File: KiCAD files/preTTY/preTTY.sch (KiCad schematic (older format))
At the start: 4 parts, among them J1 Power Bus, J2 Signal Buss

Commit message: home
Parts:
- A1: symbol USARTv2-rescue:Arduino_Nano_v3.x-MCU_Module -> preTTY-rescue:Arduino_Nano_v3.x-MCU_Module-USARTv2-rescue
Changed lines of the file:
@@
 EESchema Schematic File Version 4
-LIBS:USARTv2-cache
+LIBS:preTTY-cache
 EELAYER 30 0
 EELAYER END
@@
 Connection ~ 3500 4350
 $Comp
-L USARTv2-rescue:Arduino_Nano_v3.x-MCU_Module A1
+L preTTY-rescue:Arduino_Nano_v3.x-MCU_Module-USARTv2-rescue A1
 U 1 1 60CCDAA2
 P 7250 3700

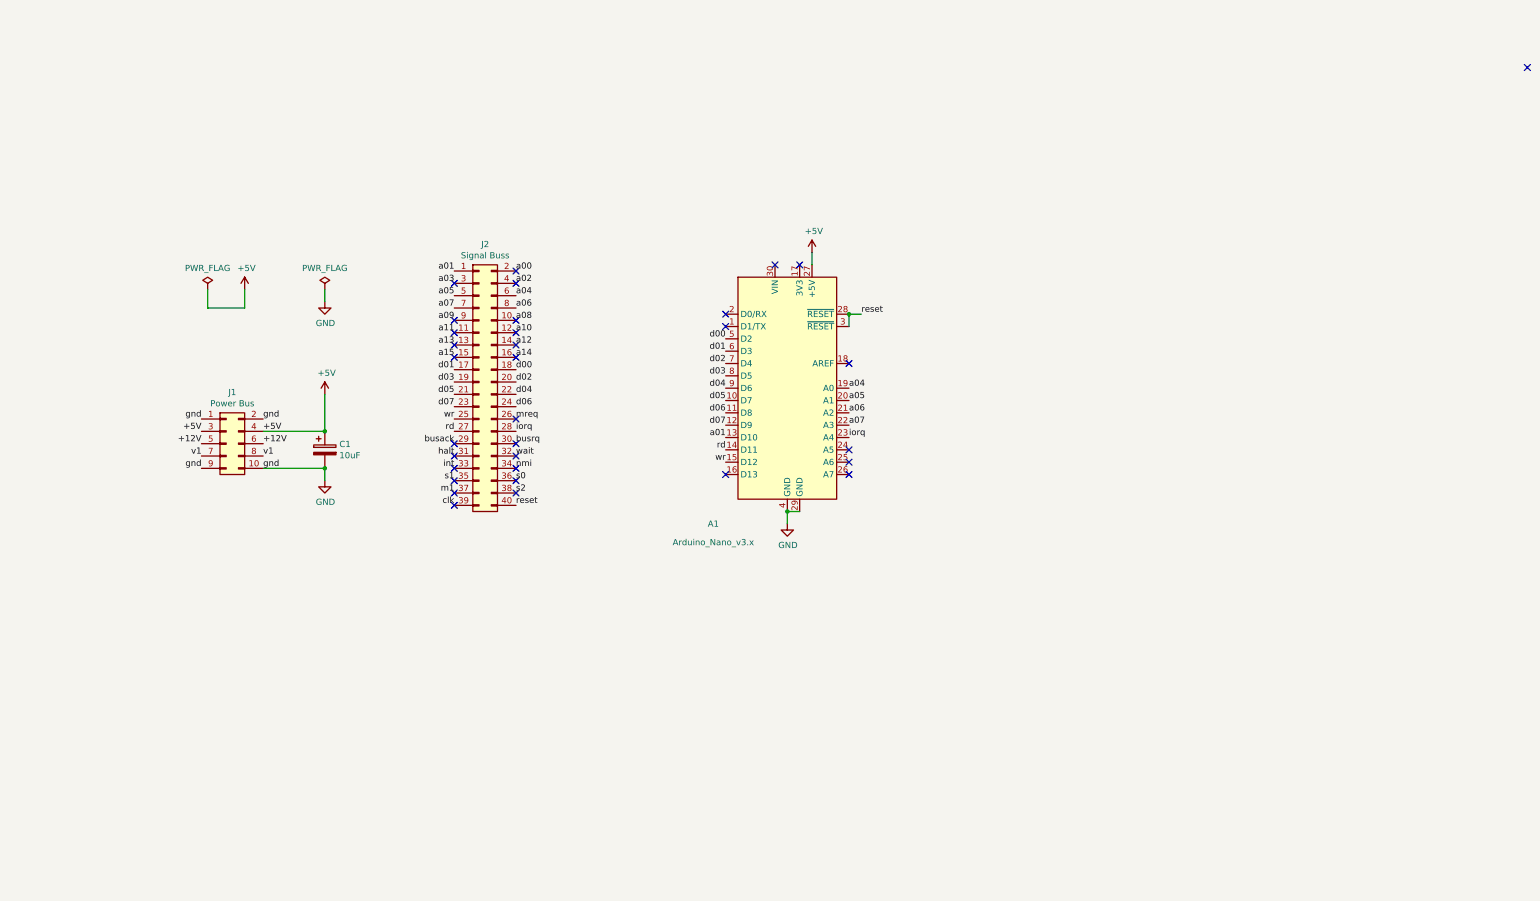
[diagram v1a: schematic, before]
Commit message: office
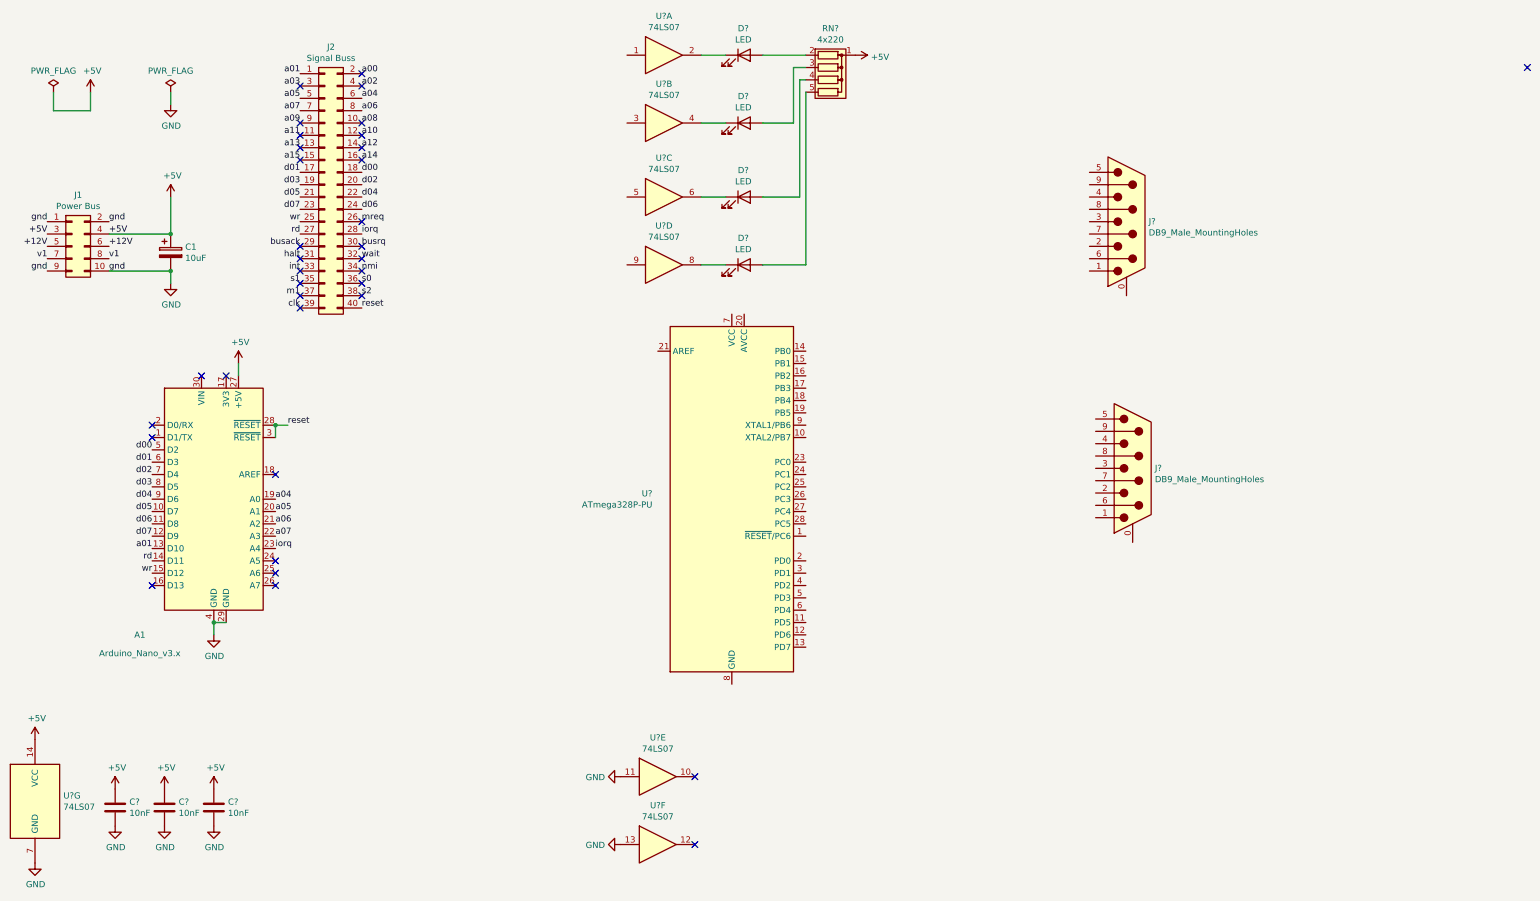
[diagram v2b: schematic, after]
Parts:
- added C? (x3): 10nF, symbol Device:C
- added D? (x4): LED, symbol Device:LED
- added J? (x2): DB9_Male_MountingHoles, symbol Connector:DB9_Male_MountingHoles
- added RN?: 4x220, Resistor_THT:R_Array_SIP5, symbol Device:R_Network04
- added U? (x7): 74LS07, symbol 74xx:74LS07
- added U?: ATmega328P-PU, Package_DIP:DIP-28_W7.62mm, symbol MCU_Microchip_ATmega:ATmega328P-PU
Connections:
- net +5V: now also C?.1, C?.1, C?.1, RN?.1 (common), U?.14 (VCC)
- net GND: now also C?.2, C?.2, C?.2, U?.11, U?.13, U?.7 (GND)
- new net: D?.1 (K), U?.2
- new net: D?.1 (K), U?.4
- new net: D?.1 (K), U?.6
- new net: D?.1 (K), U?.8
- new net: D?.2 (A), RN?.2 (R1)
- new net: D?.2 (A), RN?.3 (R2)
- new net: D?.2 (A), RN?.4 (R3)
- new net: D?.2 (A), RN?.5 (R4)
- new net: U?.22 (GND), U?.8 (GND)
- no-connect marks 33 -> 35
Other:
- moved on the sheet: A1, C1, J1, J2

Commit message: office
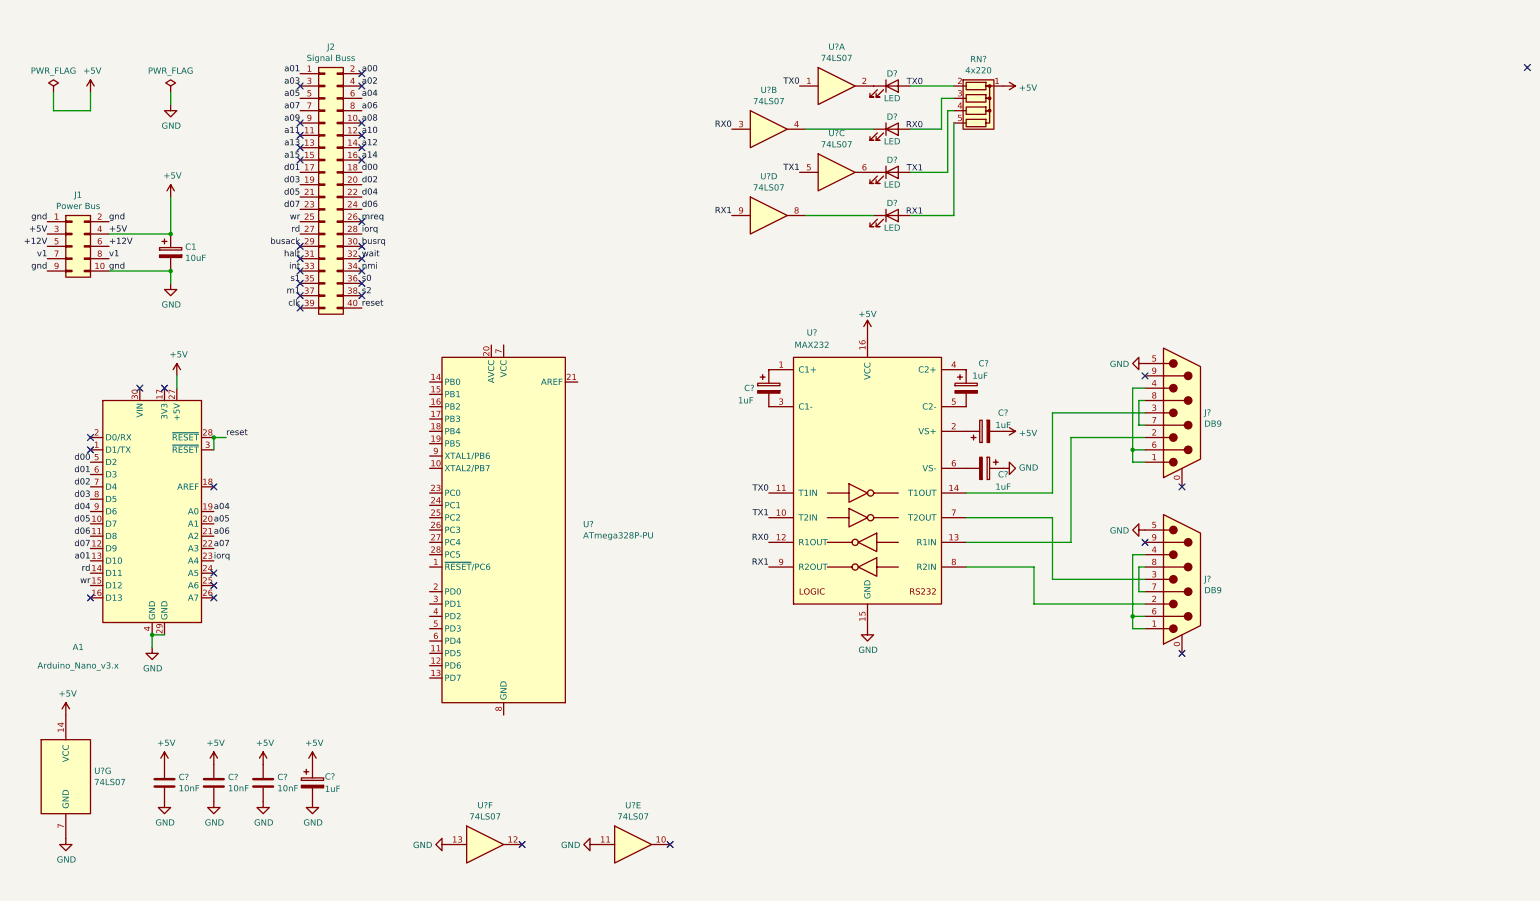
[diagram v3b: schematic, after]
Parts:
- removed J?: DB9_Male_MountingHoles, symbol Connector:DB9_Male_MountingHoles
- added C? (x5): 1uF, symbol Device:CP
- added J?: DB9, symbol Connector:DB9_Male_MountingHoles
- added U?: MAX232, symbol Interface_UART:MAX232
- J?: value DB9_Male_MountingHoles -> DB9
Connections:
- net +5V: now also C?.1, C?.2, U?.16 (VCC)
- net GND: now also J?.5, C?.1, C?.2, J?.5, U?.15 (GND)
- net TX0: now reaches U?.1
- net TX0: now also U?.11 (T1IN)
- net RX0: now reaches U?.3
- net RX0: now also U?.12 (R1OUT)
- net TX1: now reaches U?.5
- net TX1: now also U?.10 (T2IN)
- net RX1: now reaches U?.9
- net RX1: now also U?.9 (R2OUT)
- net at J?.1: now also J?.4, J?.6
- net at J?.2: now also U?.13 (R1IN)
- net at J?.3: now also U?.14 (T1OUT)
- net at J?.7: now also J?.8
- new net: C?.1, U?.1 (C1+)
- new net: C?.1, U?.2 (VS+)
- new net: C?.2, U?.3 (C1-)
- new net: C?.1, U?.4 (C2+)
- new net: C?.2, U?.5 (C2-)
- new net: C?.2, U?.6 (VS-)
- new net: J?.3, U?.7 (T2OUT)
- new net: J?.2, U?.8 (R2IN)
- new net: J?.1, J?.4, J?.6
- new net: J?.7, J?.8
- no-connect marks 35 -> 39
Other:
- note added: "RX0"
- note added: "RX1"
- note added: "TX0"
- note added: "TX1"
- moved on the sheet: A1, C?, D?, J?, RN?, U?, U?A, U?B, U?C, U?D, U?E, U?F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

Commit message: home
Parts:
- U?: symbol MCU_Microchip_ATmega:ATmega328P-PU -> preTTY-rescue:ATmega328P-PU-MCU_Microchip_ATmega
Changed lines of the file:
@@
 EESchema Schematic File Version 4
+LIBS:preTTY-cache
 EELAYER 30 0
 EELAYER END
@@
 $EndComp
 $Comp
-L MCU_Microchip_ATmega:ATmega328P-PU U?
+L preTTY-rescue:ATmega328P-PU-MCU_Microchip_ATmega U?
 U 1 1 60DFBC7C
 P 4950 4850
